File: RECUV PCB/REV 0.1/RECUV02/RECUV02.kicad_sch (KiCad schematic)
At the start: 23 parts, among them P1 VEXT, U1 ESP32-S3-WROOM-1, U2 CH340C, U3 A1117-3.3

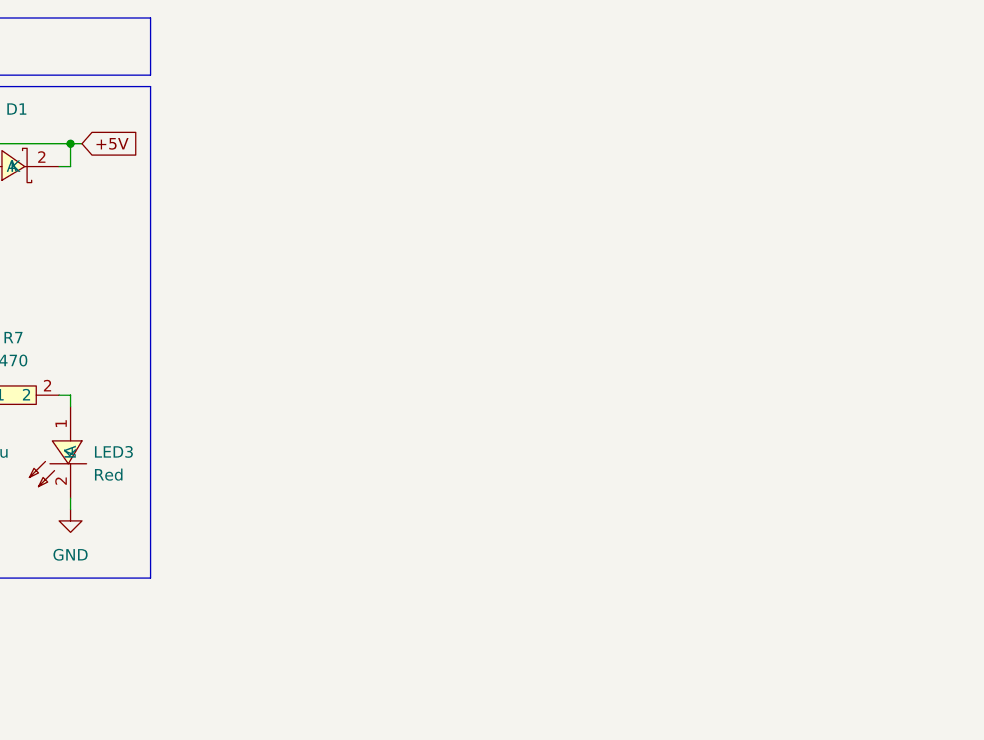
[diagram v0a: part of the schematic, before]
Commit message: Finished Boot Settings
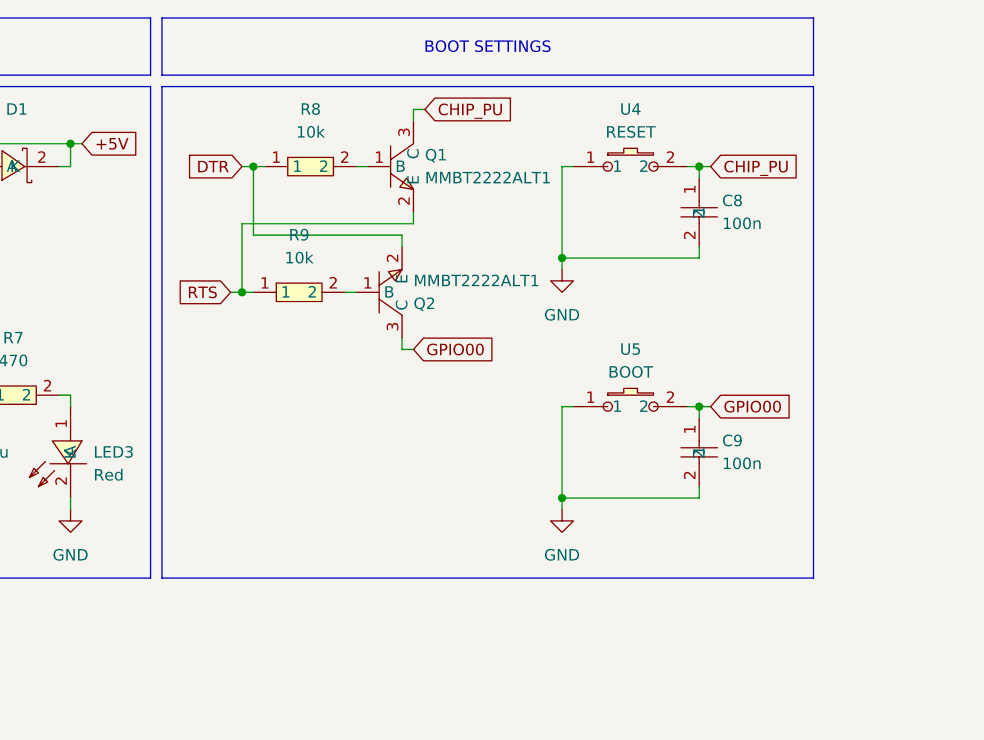
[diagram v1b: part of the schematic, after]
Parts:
- added C8, C9: 100n, EasyEDA:C0805, symbol EasyEDA:CL21B104KBCNNNC
- added Q1, Q2: MMBT2222ALT1, EasyEDA:SOT-23-3_L3.0-W1.7-P0.95-LS2.9-BR, symbol EasyEDA:MMBT2222ALT1
- added R8, R9: 10k, EasyEDA:R0805, symbol EasyEDA:0805W8F1002T5E
- added U4: RESET, EasyEDA:SW-SMD_KSR213GLFG, symbol EasyEDA:KSR213GLFG
- added U5: BOOT, EasyEDA:SW-SMD_KSR213GLFG, symbol EasyEDA:KSR213GLFG
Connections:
- net DTR: now also Q2.2 (E), R8.1
- net GND: now also C8.2, C9.2, U4.1, U5.1
- net RTS: now also Q1.2 (E), R9.1
- new net: Q1.1 (B), R8.2
- new net: Q2.1 (B), R9.2
- new net CHIP_PU: C8.1, Q1.3 (C), U4.2
- new net GPIO00: C9.1, Q2.3 (C), U5.2
